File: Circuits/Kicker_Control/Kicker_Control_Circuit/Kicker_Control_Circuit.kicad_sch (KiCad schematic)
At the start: 1 part, among them P1 66200621124

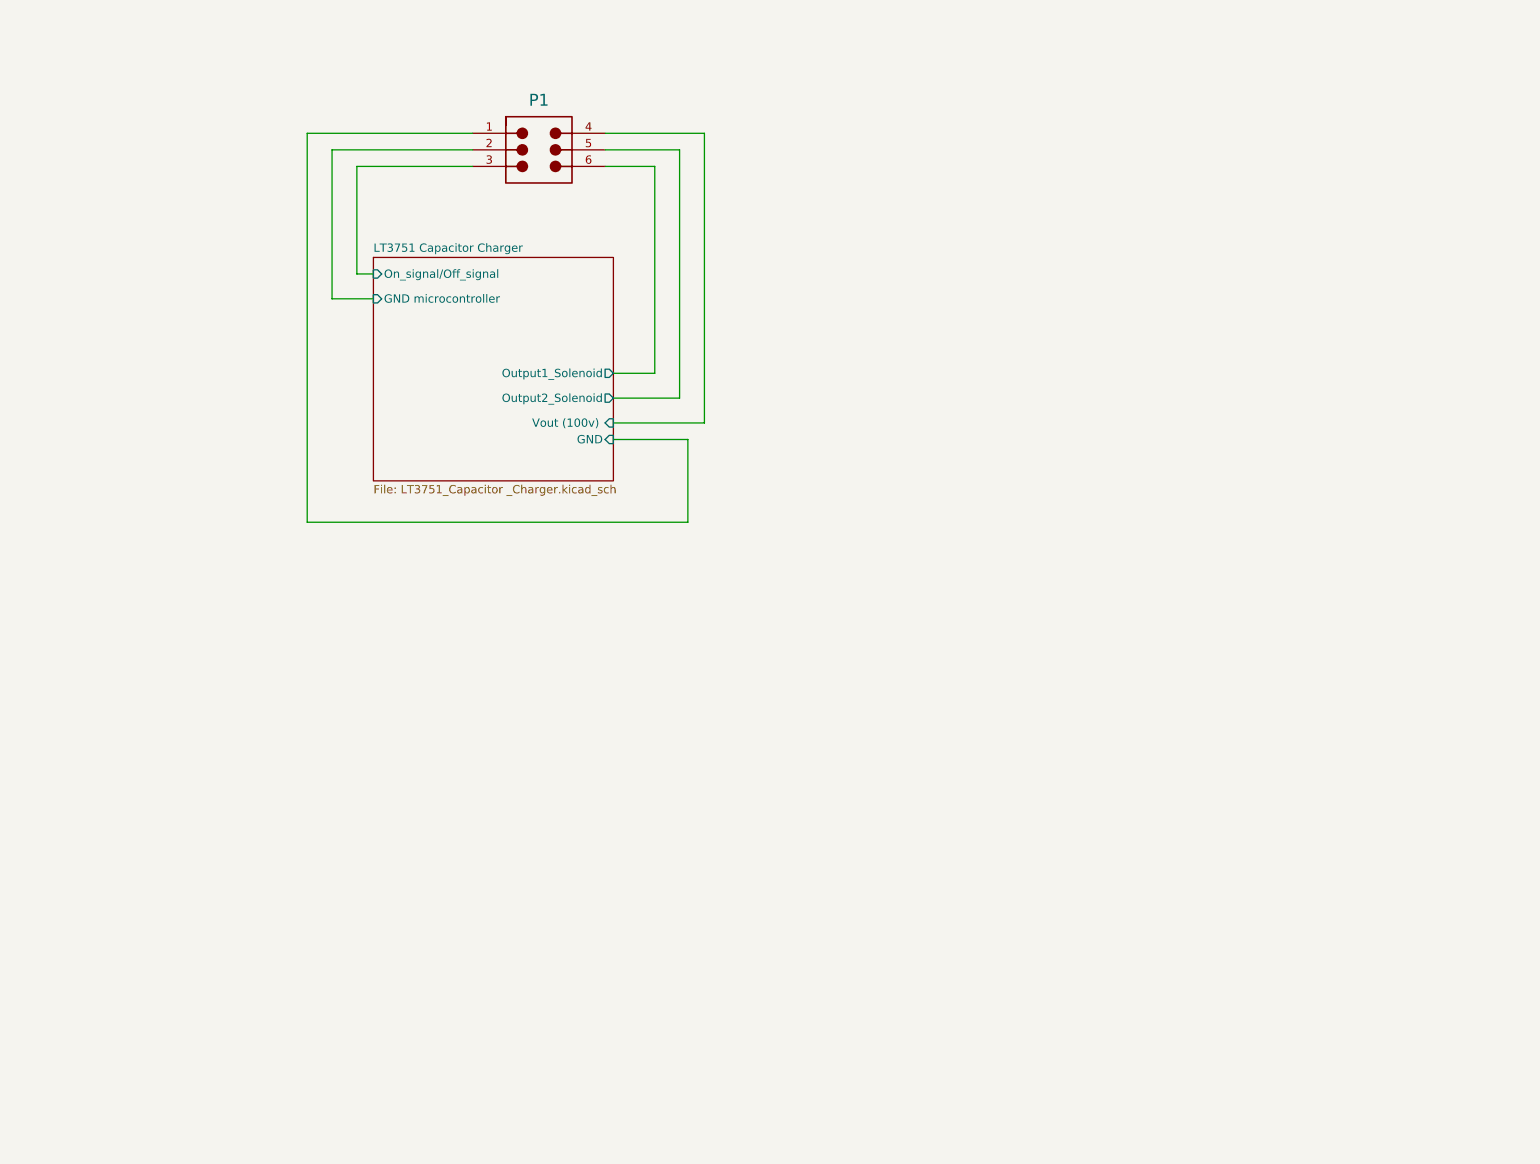
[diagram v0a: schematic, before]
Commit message: kicker circuit changest
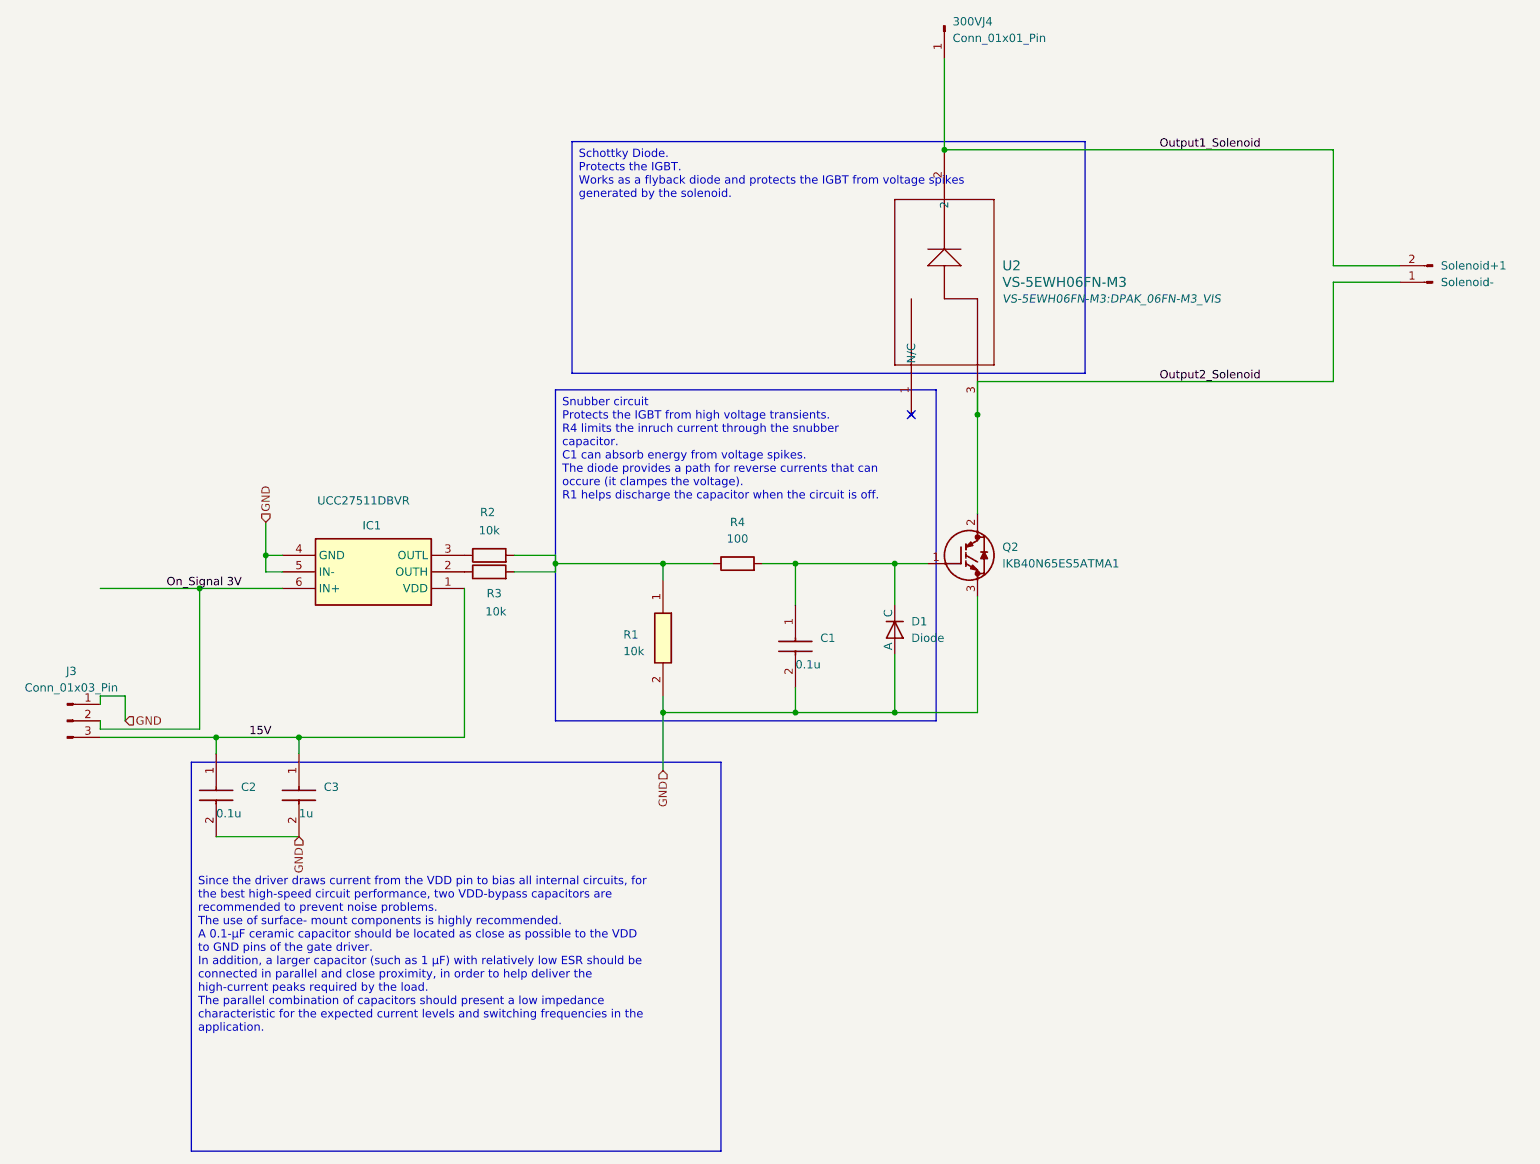
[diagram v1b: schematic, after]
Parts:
- removed P1: 66200621124, Altium_WR-MPC3 (rev23a):66200621124, symbol WR-MPC3 3.00 mm Male Header Dual Row Vertical - THT:66200621124
- added 300VJ4: Conn_01x01_Pin, Connector_PinHeader_2.54mm:PinHeader_1x01_P2.54mm_Vertical, symbol Connector:Conn_01x01_Pin
- added C1: 0.1u, Capacitor_SMD:C_1812_4532Metric, symbol B32671P6104K000:B32671P6104K000
- added C2: 0.1u, Capacitor_SMD:C_1206_3216Metric, symbol B32671P6104K000:B32671P6104K000
- added C3: 1u, Capacitor_SMD:C_1206_3216Metric, symbol B32671P6104K000:B32671P6104K000
- added D1: Diode, Diode_SMD:D_SMC, symbol TVS_Diod_1.5SMC440A:Diode
- added IC1: UCC27511DBVR, IKB40N65ES5ATMA1 IGBT:BTS141TCBUMA1, symbol UCC27511DBVR:UCC27511DBVR
- added J3: Conn_01x03_Pin, Connector_PinHeader_2.54mm:PinHeader_1x03_P2.54mm_Vertical, symbol Connector:Conn_01x03_Pin
- added Q2: IKB40N65ES5ATMA1, IKB40N65ES5ATMA1 IGBT:BTS141TCBUMA1, symbol IKB40N65ES5ATMA1:IKB40N65ES5ATMA1
- added R1: 10k, Resistor_SMD:R_1210_3225Metric, symbol CRCW121010K0JNEAIF:CRCW121010K0JNEAIF
- added R2, R3: 10k, Resistor_SMD:R_1210_3225Metric, symbol Device:R
- added R4: 100, Resistor_SMD:R_2010_5025Metric, symbol Device:R
- added Solenoid+1: Solenoid-, Connector_PinHeader_2.54mm:PinHeader_1x02_P2.54mm_Vertical, symbol Connector:Conn_01x02_Pin
- added U2: VS-5EWH06FN-M3, VS-5EWH06FN-M3:DPAK_06FN-M3_VIS, symbol VS-5EWH06FN-M3:VS-5EWH06FN-M3
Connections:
- new net: R1.1, R2.2, R3.2, R4.1
- new net: C1.1, D1.2 (C), Q2.1 (G), R4.2
- new net: IC1.2 (OUTH), R3.1
- new net: IC1.3 (OUTL), R2.1
- new net 15V: C2.1, C3.1, IC1.1 (VDD), J3.3 (Pin_3)
- new net GND: C1.2, C2.2, C3.2, D1.1 (A), IC1.4 (GND), IC1.5 (IN-), J3.1 (Pin_1), Q2.3 (E), R1.2
- new net On_Signal 3V: IC1.6 (IN+), J3.2 (Pin_2)
- new net Output1_Solenoid : 300VJ4.1 (Pin_1), Solenoid+1.2 (Pin_2), U2.2
- new net Output2_Solenoid : Q2.2 (C), Solenoid+1.1 (Pin_1), U2.3
- no-connect marks 0 -> 1
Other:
- removed sheet LT3751 Capacitor Charger
